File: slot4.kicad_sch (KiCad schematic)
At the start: 1 part

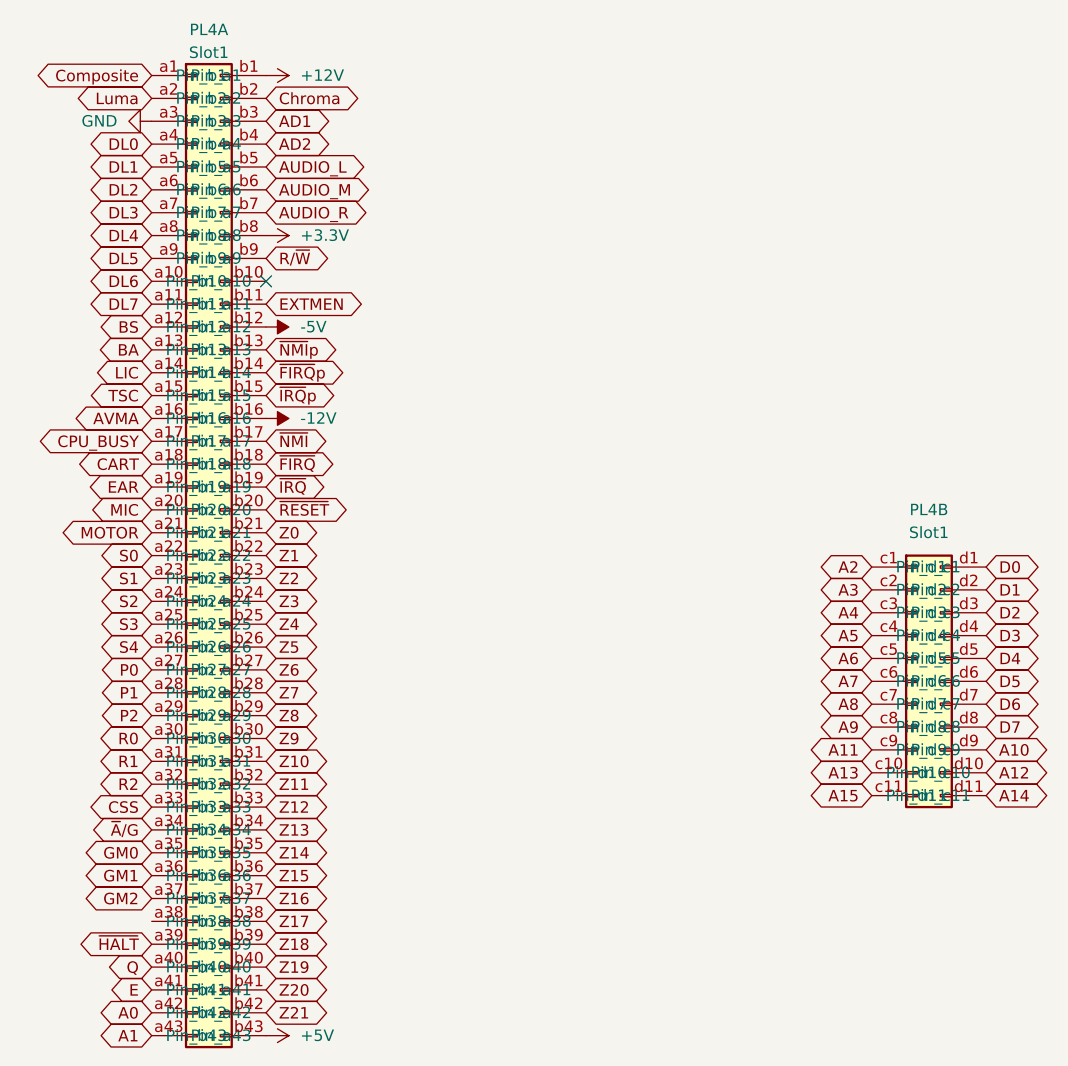
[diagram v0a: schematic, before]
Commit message: board layout
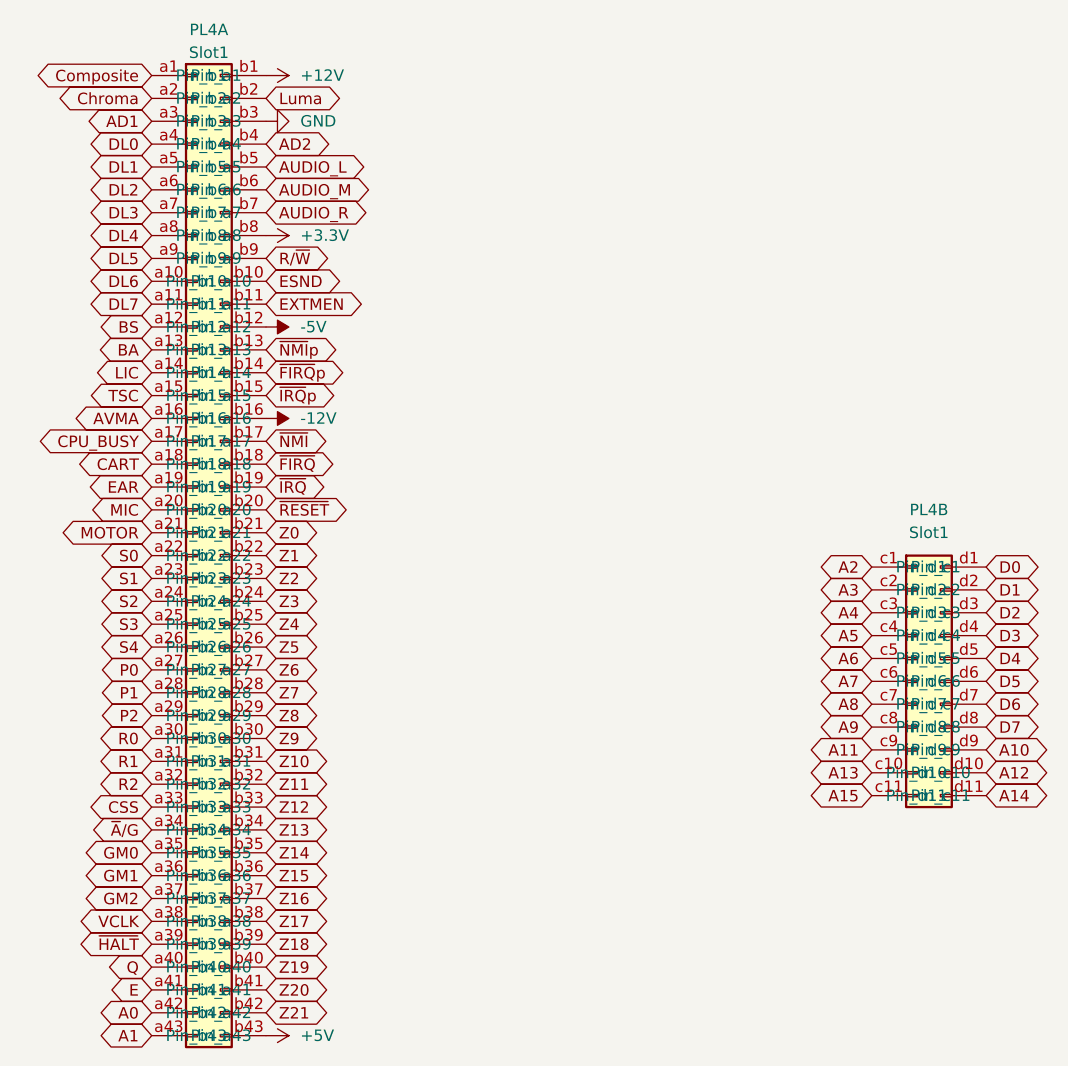
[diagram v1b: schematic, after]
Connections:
- net AD1: now also PL4.a3 (Pin_a3); no longer PL4.b3 (Pin_b3)
- net Chroma: now also PL4.a2 (Pin_a2); no longer PL4.b2 (Pin_b2)
- net GND: now also PL4.b3 (Pin_b3); no longer PL4.a3 (Pin_a3)
- net Luma: now also PL4.b2 (Pin_b2); no longer PL4.a2 (Pin_a2)
- net VCLK: now reaches PL4.a38 (Pin_a38)
- net ESND: now reaches PL4.b10 (Pin_b10)
- no-connect marks 1 -> 0
